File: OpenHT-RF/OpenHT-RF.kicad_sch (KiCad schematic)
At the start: 0 parts

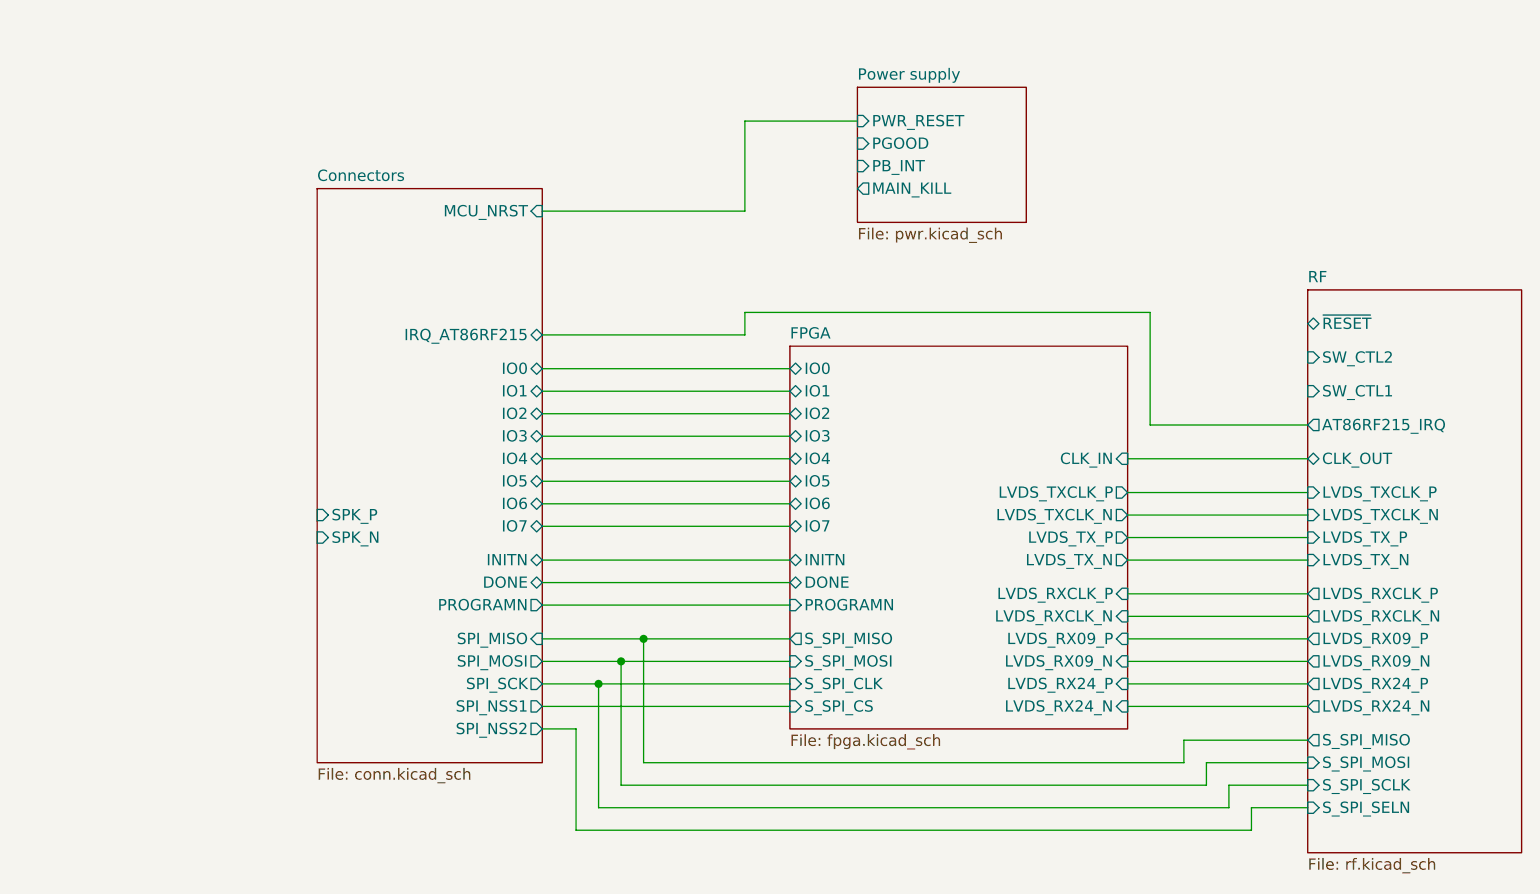
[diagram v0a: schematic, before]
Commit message: Optimised IO routing, renumbered components
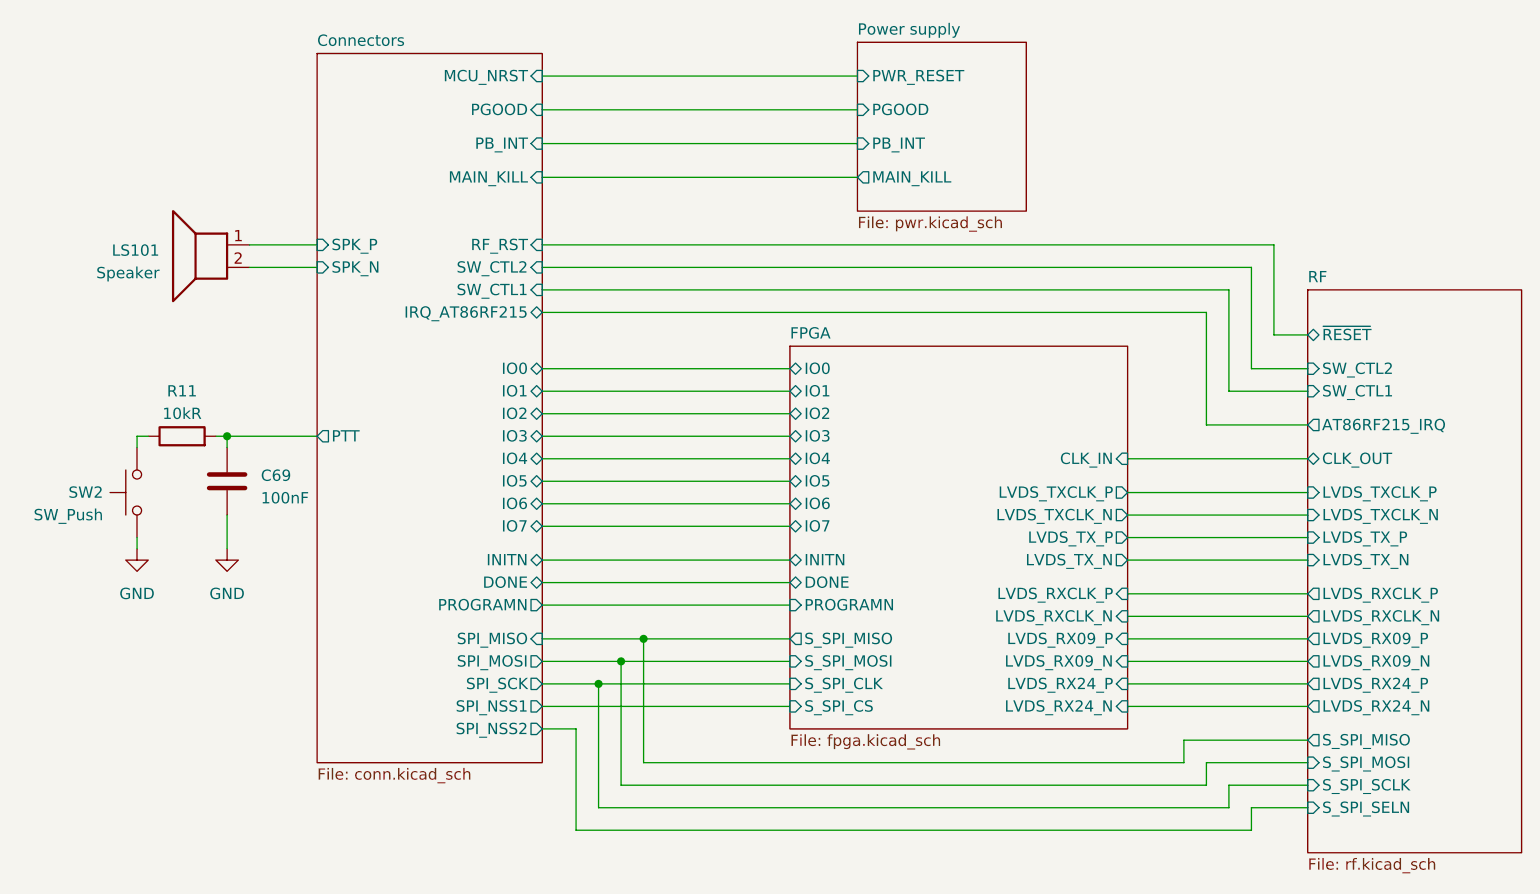
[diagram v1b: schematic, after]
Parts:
- added C69: 100nF, symbol Device:C
- added LS101: Speaker, symbol Device:Speaker
- added R11: 10kR, symbol Device:R
- added SW2: SW_Push, symbol Switch:SW_Push
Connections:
- net Connectors/SPK_N: now also LS101.2
- net Connectors/SPK_P: now also LS101.1
- new net: R11.1, SW2.2
- new net Connectors/PTT: C69.1, R11.2
- new net GND: C69.2, SW2.1
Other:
- sheet Connectors ports: added MAIN_KILL, PB_INT, PGOOD, PTT, RF_RST, SW_CTL1, SW_CTL2; removed none
